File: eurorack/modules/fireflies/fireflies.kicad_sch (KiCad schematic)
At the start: 45 parts, among them J1 Conn_01x04, J2 AudioJack2_SwitchT, J3 AudioJack2_SwitchT, J4 AudioJack2_SwitchT, J5 AudioJack2_SwitchT, SW1 SW_Push_LED, SW2 SW_Push_LED, U1 MIC5219-5.0YM5, U2 Chordata, U3 MCP4822, U4 TLC5971PWP

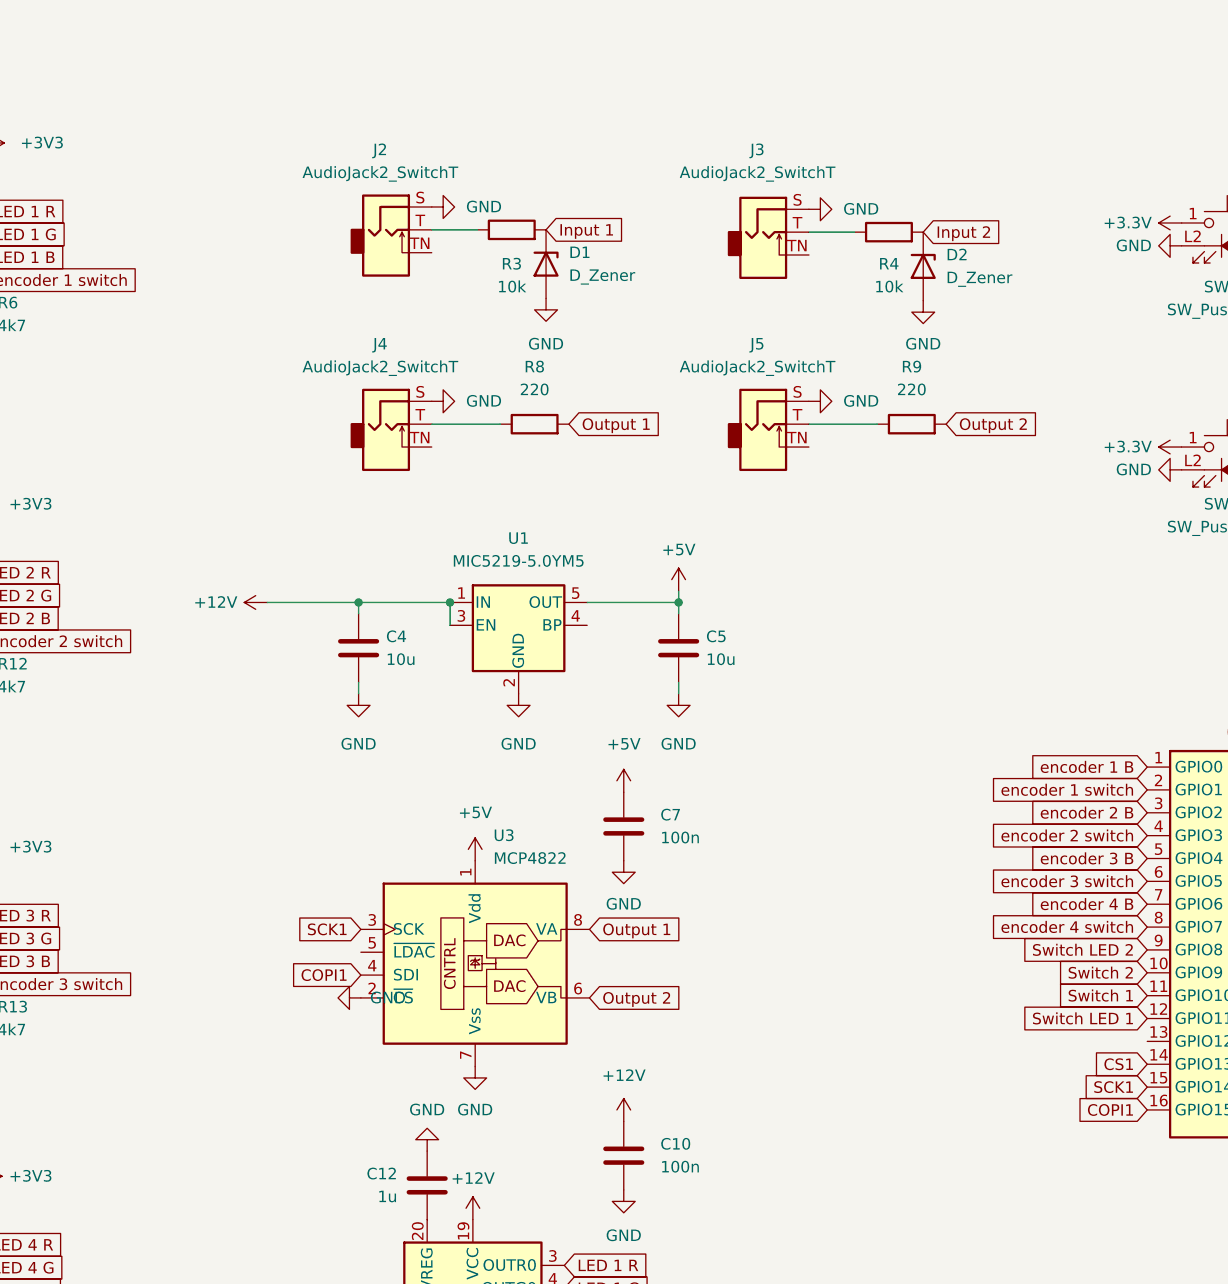
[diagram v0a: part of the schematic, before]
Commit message: i honestly have no idea
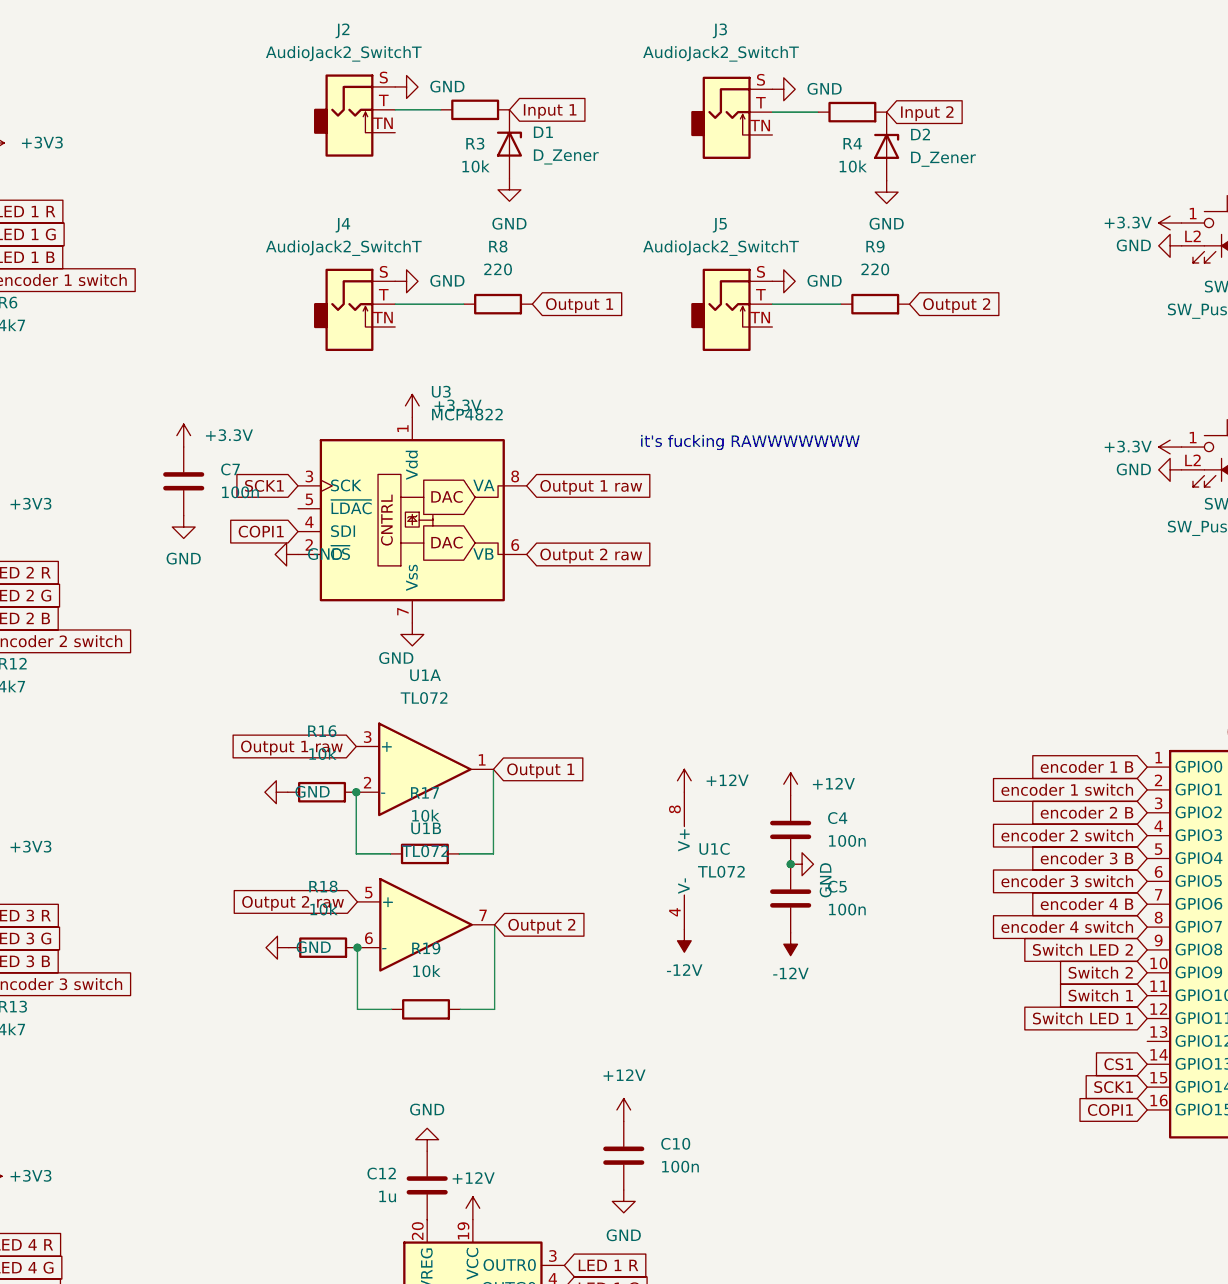
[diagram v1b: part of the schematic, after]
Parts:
- removed U1: MIC5219-5.0YM5, Package_TO_SOT_SMD:SOT-23-5, symbol Regulator_Linear:MIC5219-5.0YM5
- added R16, R17, R18, R19: 10k, Resistor_SMD:R_0805_2012Metric_Pad1.20x1.40mm_HandSolder, symbol Device:R
- added U1: TL072, symbol Amplifier_Operational:TL072
- C4, C5: value 10u -> 100n
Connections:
- net +12V: now also C4.2, U1.8 (V+); no longer C4.1
- net +3V3: now also C7.2, U3.1 (Vdd)
- net -12V: now also C5.1, U1.4 (V-)
- net GND: now also C4.1, R16.1, R18.1; no longer C4.2
- net Output 1: now also R17.2, U1.1; no longer U3.8 (VA)
- net Output 2: now also R19.2, U1.7; no longer U3.6 (VB)
- removed net +5V: C5.1, C7.2, U3.1 (Vdd)
- new net: R18.2, R19.1, U1.6 (-)
- new net: R16.2, R17.1, U1.2 (-)
- new net Output 1 raw: U1.3 (+), U3.8 (VA)
- new net Output 2 raw: U1.5 (+), U3.6 (VB)
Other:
- note added: "it's fucking RAWWWWWWW"
- moved on the sheet: C7, D1, D2, J2, J3, J4, J5, R3, R4, R8, R9, U3
